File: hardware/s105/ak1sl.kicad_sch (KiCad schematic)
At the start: 15 parts, among them Q18 BC847C, Q8 BC847C, U1 case only

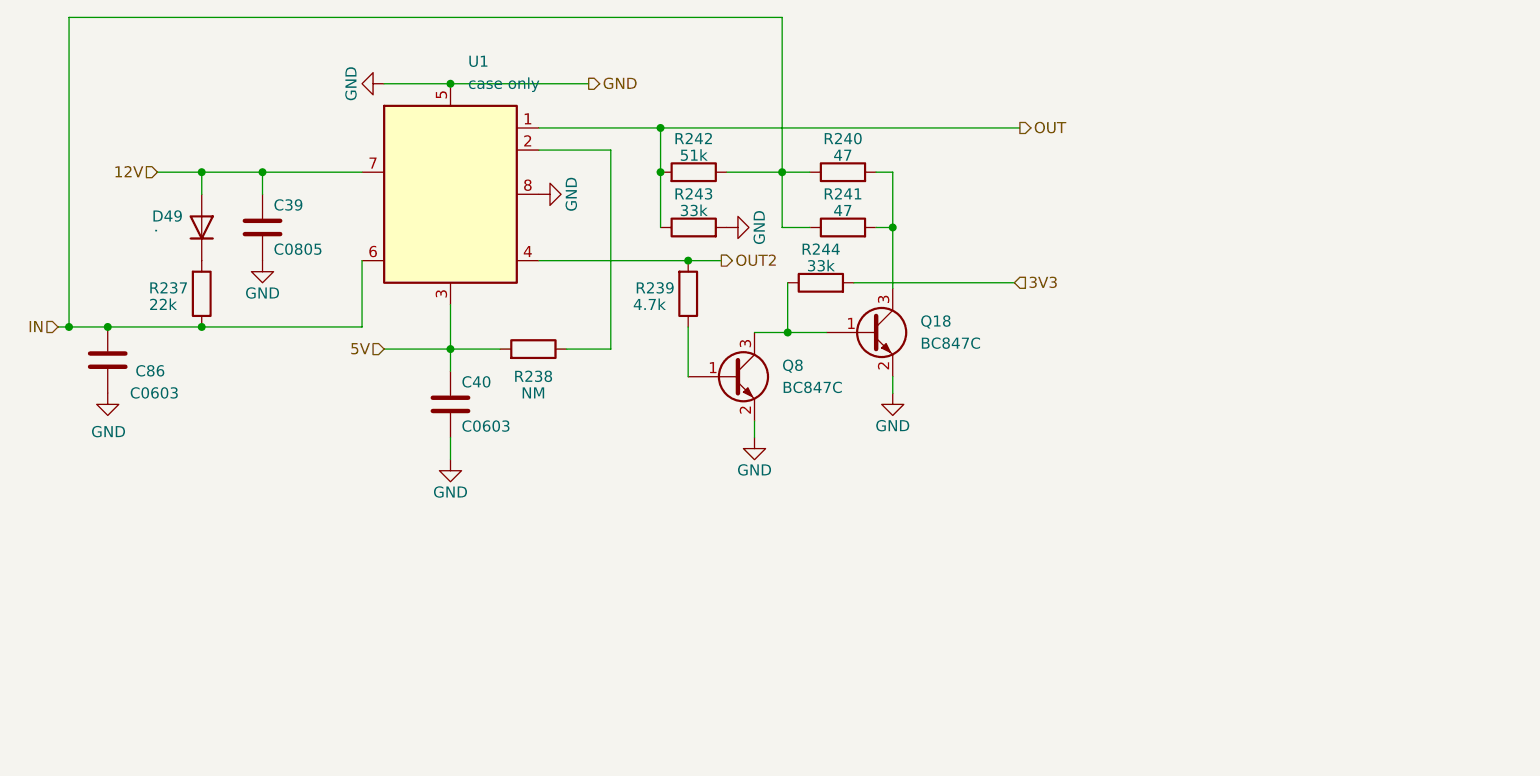
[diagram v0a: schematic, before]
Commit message: заполняем плату дальше
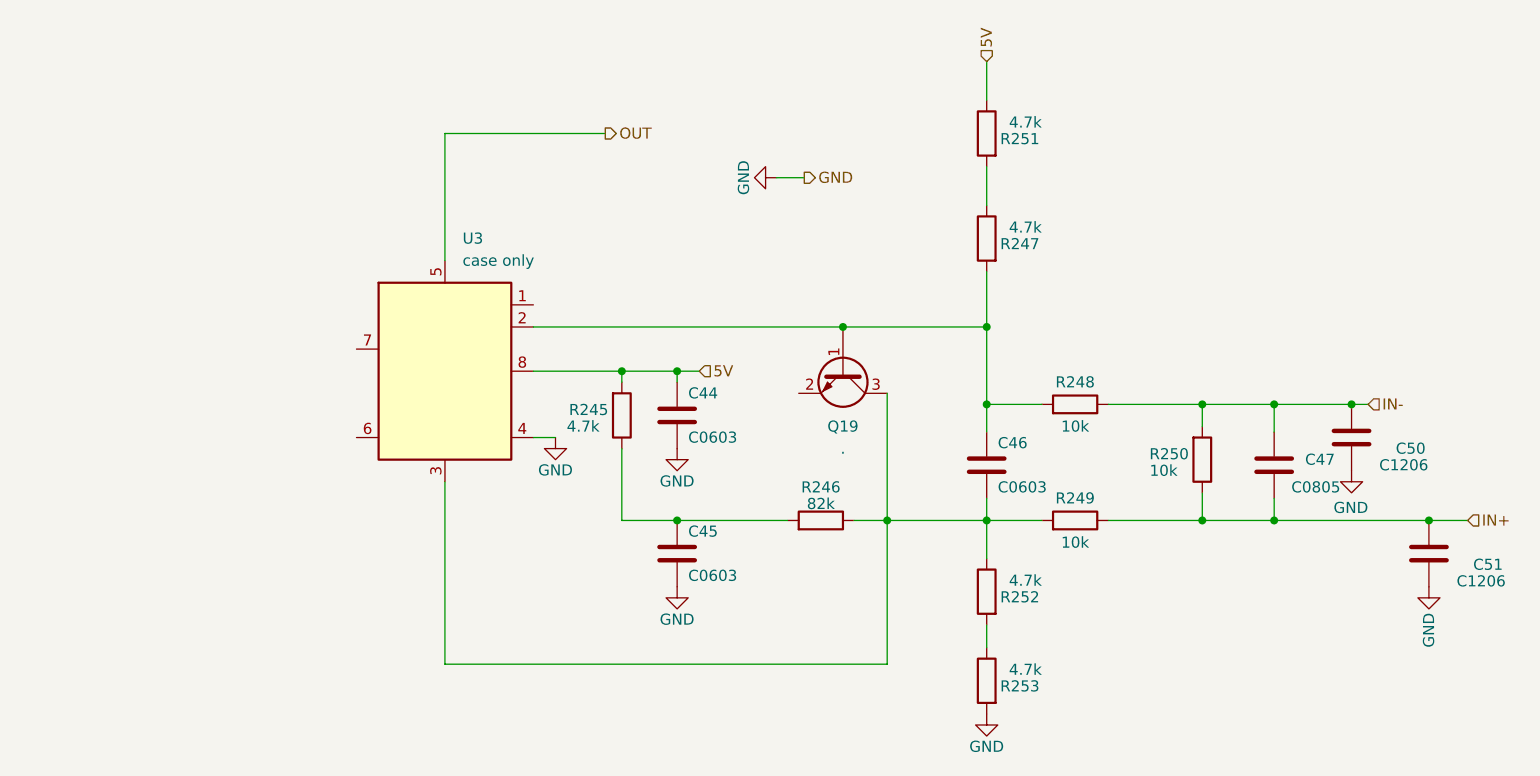
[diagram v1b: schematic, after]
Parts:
- removed C39: C0805, Capacitor_SMD:C_0805_2012Metric, symbol Device:C
- removed C40, C86: C0603, Capacitor_SMD:C_0603_1608Metric, symbol Device:C
- removed D49: ., Diode_SMD:D_SOD-123, symbol Diode:1N4148W
- removed Q18, Q8: BC847C, Package_TO_SOT_SMD:SOT-23, symbol Transistor_BJT:BC847
- removed R237: 22k, Resistor_SMD:R_0603_1608Metric, symbol Device:R
- removed R238: NM, Resistor_SMD:R_0603_1608Metric, symbol Device:R
- removed R239: 4.7k, Resistor_SMD:R_0603_1608Metric, symbol Device:R
- removed R240, R241: 47, Resistor_SMD:R_0603_1608Metric, symbol Device:R
- removed R242: 51k, Resistor_SMD:R_0603_1608Metric, symbol Device:R
- removed R243, R244: 33k, Resistor_SMD:R_0603_1608Metric, symbol Device:R
- removed U1: case only, Package_SO:SOIC-8_3.9x4.9mm_P1.27mm, symbol Regulator_Controller:L6727
- added C44, C45, C46: C0603, Capacitor_SMD:C_0603_1608Metric, symbol Device:C
- added C47: C0805, Capacitor_SMD:C_0805_2012Metric, symbol Device:C
- added C50, C51: C1206, Capacitor_SMD:C_1206_3216Metric, symbol Device:C
- added Q19: ., Package_TO_SOT_SMD:SOT-23, symbol Transistor_BJT:BC847
- added R245, R247, R251, R252, R253: 4.7k, Resistor_SMD:R_0603_1608Metric, symbol Device:R
- added R246: 82k, Resistor_SMD:R_0603_1608Metric, symbol Device:R
- added R248, R249, R250: 10k, Resistor_SMD:R_0805_2012Metric, symbol Device:R
- added U3: case only, Package_SO:SOIC-8_3.9x4.9mm_P1.27mm, symbol Regulator_Controller:L6727
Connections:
- net 5V: now also C44.1, R245.2, R251.1, U3.8 (PHASE)
- net GND: now also C44.2, C45.2, C50.2, C51.2, R253.2, U3.4 (LGATE)
- net OUT: now also U3.5 (VCC)
- new net: R252.2, R253.1
- new net: C46.1, Q19.1 (B), R247.2, R248.2, U3.2 (UGATE)
- new net: C45.1, R245.1, R246.2
- new net: C46.2, Q19.3 (C), R246.1, R249.2, R252.1, U3.3 (GND)
- new net: R247.1, R251.2
- new net IN+: C47.1, C51.1, R249.1, R250.1
- new net IN-: C47.2, C50.1, R248.1, R250.2
